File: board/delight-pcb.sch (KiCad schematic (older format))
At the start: 171 parts, among them J1 AVR-ISP-6, SW0 KEYSW, SW1 KEYSW, SW10 KEYSW, SW11 KEYSW, SW12 KEYSW, SW13 KEYSW, SW14 KEYSW, SW15 KEYSW, SW16 KEYSW, SW17 KEYSW, SW18 KEYSW, SW19 KEYSW, SW2 KEYSW, SW20 KEYSW, SW21 KEYSW, SW22 KEYSW, SW23 KEYSW, SW24 KEYSW, SW25 KEYSW, SW26 KEYSW, SW27 KEYSW, SW28 KEYSW, SW28-2 KEYSW, SW29 KEYSW, SW3 KEYSW, SW30 KEYSW, SW31 KEYSW, SW32 KEYSW, SW33 KEYSW, SW34 KEYSW, SW35 KEYSW, SW36 KEYSW, SW37 KEYSW, SW38 KEYSW, SW39 KEYSW, SW4 KEYSW, SW40 KEYSW, SW41 KEYSW, SW42 KEYSW, SW42-2 KEYSW, SW43 KEYSW, SW44 KEYSW, SW44-2 KEYSW, SW45 KEYSW, SW46 KEYSW, SW47 KEYSW, SW48 KEYSW, SW49 KEYSW, SW5 KEYSW, SW50 KEYSW, SW51 KEYSW, SW52 KEYSW, SW53 KEYSW, SW54 KEYSW, SW55 KEYSW, SW56 KEYSW, SW57 KEYSW, SW58 KEYSW, SW59 KEYSW, SW59-2 KEYSW, SW6 KEYSW, SW60 KEYSW, SW60-2 KEYSW, SW61 KEYSW, SW62-2 KEYSW, SW63 KEYSW, SW63-2 KEYSW, SW64 KEYSW, SW64-2 KEYSW, SW65 KEYSW, SW65-2 KEYSW, SW66 KEYSW, SW67 KEYSW, SW68 KEYSW, SW69 KEYSW, SW7 KEYSW, SW8 KEYSW, SW9 KEYSW, U1 ATmega32A-PU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

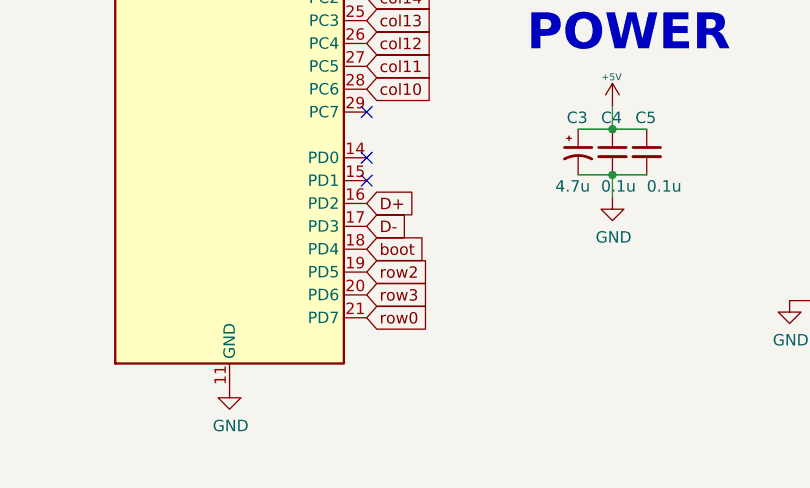
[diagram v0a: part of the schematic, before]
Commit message: Updated all routes.
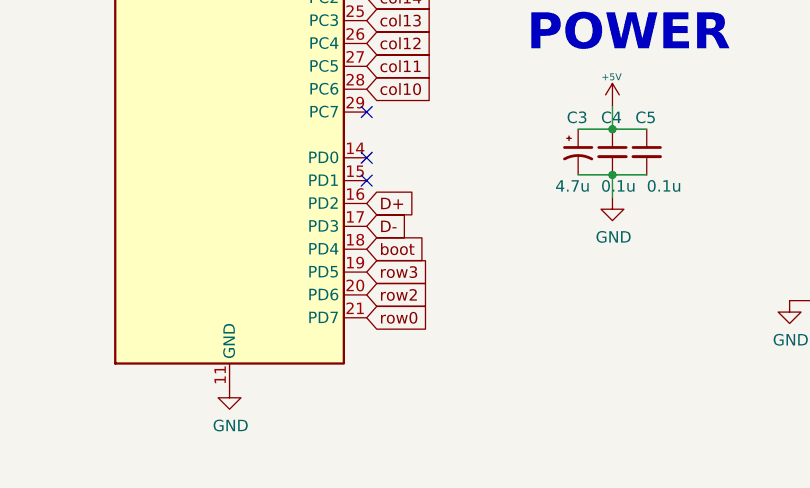
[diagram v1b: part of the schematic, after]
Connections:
- net row2: now also U1.20 (PD6); no longer U1.19 (PD5)
- net row3: now also U1.19 (PD5); no longer U1.20 (PD6)
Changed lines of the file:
@@
 Text GLabel 4575 8900 2    50   Input ~ 0
 row4
-Text GLabel 4575 10300 2    50   Input ~ 0
+Text GLabel 4575 10200 2    50   Input ~ 0
 row3
 Text GLabel 4575 10400 2    50   Input ~ 0
@@
 Text GLabel 4575 8800 2    50   Input ~ 0
 row1
-Text GLabel 4575 10200 2    50   Input ~ 0
+Text GLabel 4575 10300 2    50   Input ~ 0
 row2
 $EndSCHEMATC

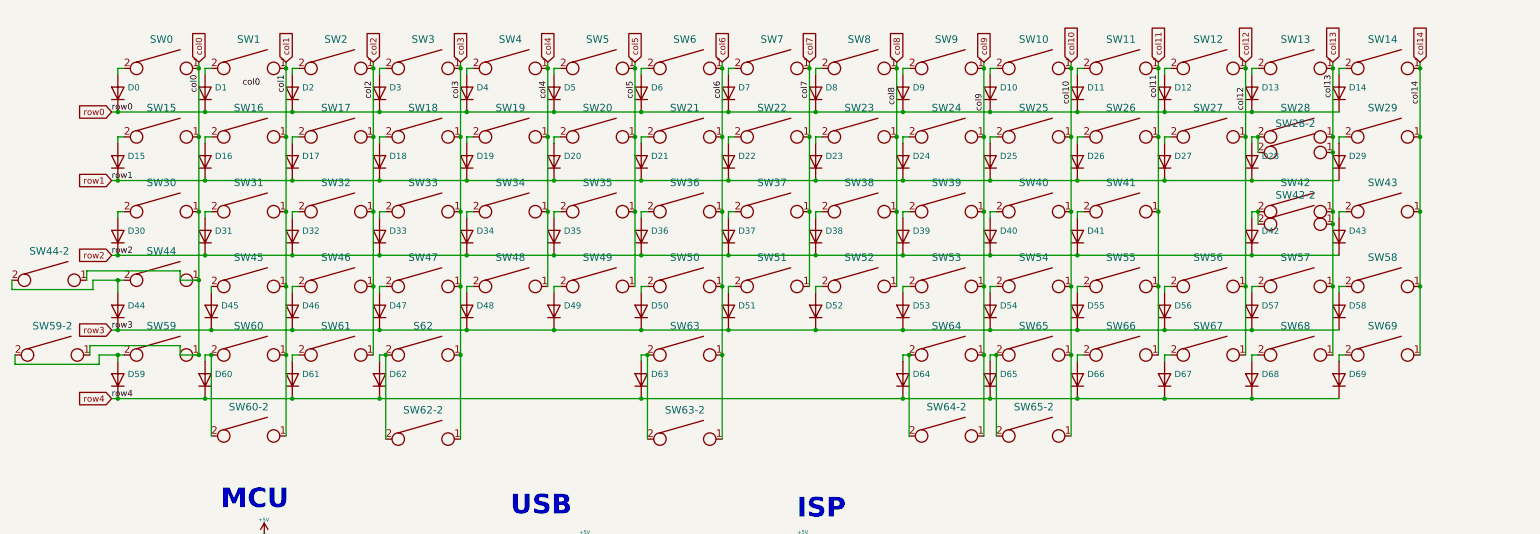
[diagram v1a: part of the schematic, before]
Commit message: More cleanup
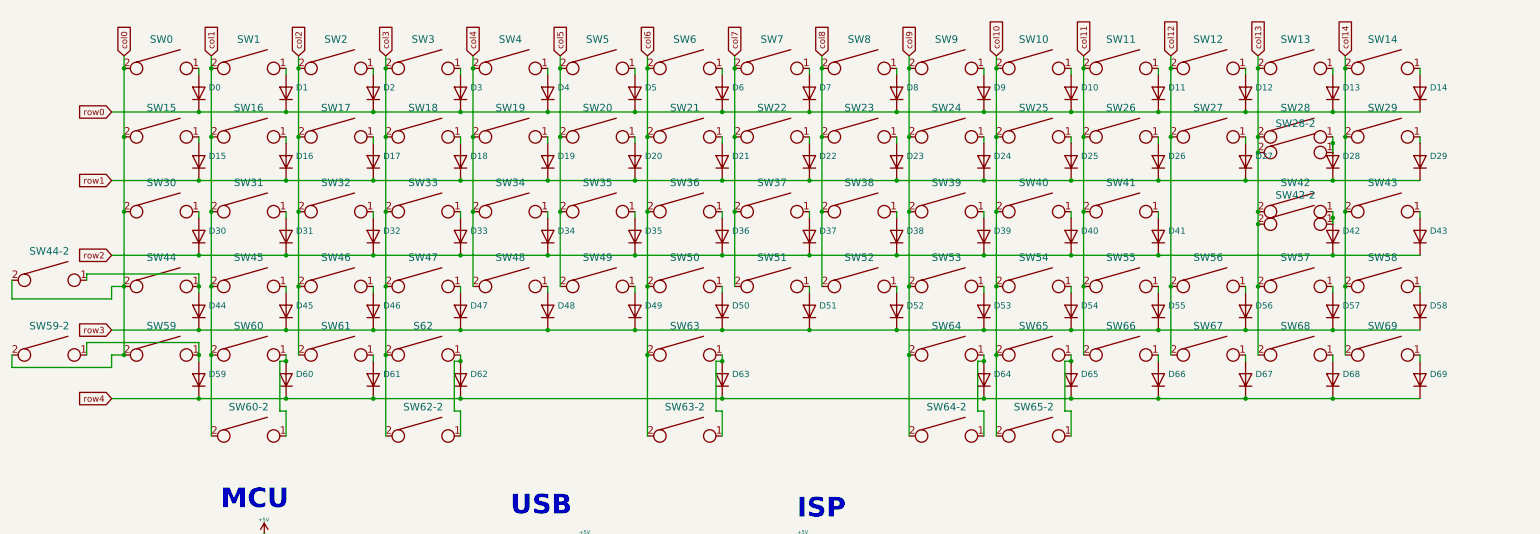
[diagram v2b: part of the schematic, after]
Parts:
- S62, SW44-2, SW59-2, SW60, SW61, SW64, SW65: footprint cftkb:SW_Cherry_MX1A_1.25u_PCBNOSCREEN -> cherrymx:SW_Cherry_MX_PCB_1.25u
- SW0, SW1, SW10, SW11, SW12, SW14, SW15, SW16, SW17, SW18, SW19, SW2, SW20, SW21, SW22, SW23, SW24, SW25, SW26, SW27, SW29, SW3, SW31, SW32, SW33, SW34, SW35, SW36, SW37, SW38, SW39, SW4, SW40, SW41, SW42-2, SW43, SW45, SW46, SW47, SW48, SW49, SW5, SW50, SW51, SW52, SW53, SW54, SW55, SW57, SW58, SW6, SW63, SW63-2, SW66, SW67, SW68, SW69, SW7, SW8, SW9: footprint cftkb:SW_Cherry_MX1A_1.00u_PCB-NOSCREEN -> cherrymx:SW_Cherry_MX_PCB_1.00u
- SW13: footprint cftkb:SW_Cherry_MX1A_2.00u_PCBNOSCREEN -> cherrymx:SW_Cherry_MX_PCB_2.00u
- SW28, SW30, SW60-2, SW62-2, SW64-2, SW65-2: footprint cftkb:SW_Cherry_MX1A_1.50u_PCBNOSCREEN -> cherrymx:SW_Cherry_MX_PCB_1.50u
- SW28-2: footprint cftkb:SW_Cherry_MX1A_ISOEnter_PCB_ReversedStabilizer -> cherrymx:SW_Cherry_MX_Plate_ISOEnter
- SW42, SW59: footprint cftkb:SW_Cherry_MX1A_2.25u_PCBNOSCREEN -> cherrymx:SW_Cherry_MX_PCB_2.25u
- SW44, SW56: footprint cftkb:SW_Cherry_MX1A_1.75u_PCBNOSCREEN -> cherrymx:SW_Cherry_MX_PCB_1.75u
- U1: footprint cftkb:DIP-40_W15.24mm -> Package_DIP:DIP-40_W15.24mm
- USB1: footprint cftkb:USB_C_GCT_USB4085 -> Connector_USB:USB_C_Receptacle_GCT_USB4085
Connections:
- net col0: now also SW0.2, SW15.2, SW30.2, SW44-2.2, SW44.2, SW59-2.2, SW59.2; no longer SW0.1, SW15.1, SW30.1, SW44-2.1, SW44.1, SW59-2.1, SW59.1
- net col1: now also SW1.2, SW16.2, SW31.2, SW45.2, SW60-2.2, SW60.2; no longer SW1.1, SW16.1, SW31.1, SW45.1, SW60-2.1, SW60.1
- net col10: now also SW10.2, SW25.2, SW40.2, SW54.2, SW65-2.2, SW65.2; no longer SW10.1, SW25.1, SW40.1, SW54.1, SW65-2.1, SW65.1
- net col11: now also SW11.2, SW26.2, SW41.2, SW55.2, SW66.2; no longer SW11.1, SW26.1, SW41.1, SW55.1, SW66.1
- net col12: now also SW12.2, SW27.2, SW56.2, SW67.2; no longer SW12.1, SW27.1, SW56.1, SW67.1
- net col13: now also SW13.2, SW28-2.2, SW28.2, SW42-2.2, SW42.2, SW57.2, SW68.2; no longer SW13.1, SW28-2.1, SW28.1, SW42-2.1, SW42.1, SW57.1, SW68.1
- net col14: now also SW14.2, SW29.2, SW43.2, SW58.2, SW69.2; no longer SW14.1, SW29.1, SW43.1, SW58.1, SW69.1
- net col2: now also SW17.2, SW2.2, SW32.2, SW46.2, SW61.2; no longer SW17.1, SW2.1, SW32.1, SW46.1, SW61.1
- net col3: now also S62.2, SW18.2, SW3.2, SW33.2, SW47.2, SW62-2.2; no longer S62.1, SW18.1, SW3.1, SW33.1, SW47.1, SW62-2.1
- net col4: now also SW19.2, SW34.2, SW4.2, SW48.2; no longer SW19.1, SW34.1, SW4.1, SW48.1
- net col5: now also SW20.2, SW35.2, SW49.2, SW5.2; no longer SW20.1, SW35.1, SW49.1, SW5.1
- net col6: now also SW21.2, SW36.2, SW50.2, SW6.2, SW63-2.2, SW63.2; no longer SW21.1, SW36.1, SW50.1, SW6.1, SW63-2.1, SW63.1
- net col7: now also SW22.2, SW37.2, SW51.2, SW7.2; no longer SW22.1, SW37.1, SW51.1, SW7.1
- net col8: now also SW23.2, SW38.2, SW52.2, SW8.2; no longer SW23.1, SW38.1, SW52.1, SW8.1
- net col9: now also SW24.2, SW39.2, SW53.2, SW64-2.2, SW64.2, SW9.2; no longer SW24.1, SW39.1, SW53.1, SW64-2.1, SW64.1, SW9.1
- net at D15.2 (A): now also SW15.1; no longer SW15.2
- net at D1.2 (A): now also SW1.1; no longer SW1.2
- net at D2.2 (A): now also SW2.1; no longer SW2.2
- net at D3.2 (A): now also SW3.1; no longer SW3.2
- net at D4.2 (A): now also SW4.1; no longer SW4.2
- net at D5.2 (A): now also SW5.1; no longer SW5.2
- net at D6.2 (A): now also SW6.1; no longer SW6.2
- net at D7.2 (A): now also SW7.1; no longer SW7.2
- net at D8.2 (A): now also SW8.1; no longer SW8.2
- net at D9.2 (A): now also SW9.1; no longer SW9.2
- net at D10.2 (A): now also SW10.1; no longer SW10.2
- net at D11.2 (A): now also SW11.1; no longer SW11.2
- net at D12.2 (A): now also SW12.1; no longer SW12.2
- net at D13.2 (A): now also SW13.1; no longer SW13.2
- net at D14.2 (A): now also SW14.1; no longer SW14.2
- net at D30.2 (A): now also SW30.1; no longer SW30.2
- net at D16.2 (A): now also SW16.1; no longer SW16.2
- net at D17.2 (A): now also SW17.1; no longer SW17.2
- net at D18.2 (A): now also SW18.1; no longer SW18.2
- net at D19.2 (A): now also SW19.1; no longer SW19.2
- net at D20.2 (A): now also SW20.1; no longer SW20.2
- net at D21.2 (A): now also SW21.1; no longer SW21.2
- net at D22.2 (A): now also SW22.1; no longer SW22.2
- net at D23.2 (A): now also SW23.1; no longer SW23.2
- net at D24.2 (A): now also SW24.1; no longer SW24.2
- net at D25.2 (A): now also SW25.1; no longer SW25.2
- net at D26.2 (A): now also SW26.1; no longer SW26.2
- net at D27.2 (A): now also SW27.1; no longer SW27.2
- net at D29.2 (A): now also SW29.1; no longer SW29.2
- net at D31.2 (A): now also SW31.1; no longer SW31.2
- net at D32.2 (A): now also SW32.1; no longer SW32.2
- net at D33.2 (A): now also SW33.1; no longer SW33.2
- net at D34.2 (A): now also SW34.1; no longer SW34.2
- net at D35.2 (A): now also SW35.1; no longer SW35.2
- net at D36.2 (A): now also SW36.1; no longer SW36.2
- net at D37.2 (A): now also SW37.1; no longer SW37.2
- net at D38.2 (A): now also SW38.1; no longer SW38.2
- net at D39.2 (A): now also SW39.1; no longer SW39.2
- net at D40.2 (A): now also SW40.1; no longer SW40.2
- net at D41.2 (A): now also SW41.1; no longer SW41.2
- net at D43.2 (A): now also SW43.1; no longer SW43.2
- net at D46.2 (A): now also SW46.1; no longer SW46.2
- net at D47.2 (A): now also SW47.1; no longer SW47.2
- net at D48.2 (A): now also SW48.1; no longer SW48.2
- net at D49.2 (A): now also SW49.1; no longer SW49.2
- net at D50.2 (A): now also SW50.1; no longer SW50.2
- net at D51.2 (A): now also SW51.1; no longer SW51.2
- net at D52.2 (A): now also SW52.1; no longer SW52.2
- net at D53.2 (A): now also SW53.1; no longer SW53.2
- net at D54.2 (A): now also SW54.1; no longer SW54.2
- net at D55.2 (A): now also SW55.1; no longer SW55.2
- net at D56.2 (A): now also SW56.1; no longer SW56.2
- net at D57.2 (A): now also SW57.1; no longer SW57.2
- net at D58.2 (A): now also SW58.1; no longer SW58.2
- net at D61.2 (A): now also SW61.1; no longer SW61.2
- net at D67.2 (A): now also SW67.1; no longer SW67.2
- net at D68.2 (A): now also SW68.1; no longer SW68.2
- net at D69.2 (A): now also SW69.1; no longer SW69.2
- net at D66.2 (A): now also SW66.1; no longer SW66.2
- net at D45.2 (A): now also SW45.1; no longer SW45.2
- net at D0.2 (A): now also SW0.1; no longer SW0.2
- new net: D28.2 (A), SW28-2.1, SW28.1
- new net: D44.2 (A), SW44-2.1, SW44.1
- new net: D42.2 (A), SW42-2.1, SW42.1
- new net: D59.2 (A), SW59-2.1, SW59.1
- new net: D60.2 (A), SW60-2.1, SW60.1
- new net: D62.2 (A), S62.1, SW62-2.1
- new net: D63.2 (A), SW63-2.1, SW63.1
- new net: D64.2 (A), SW64-2.1, SW64.1
- new net: D65.2 (A), SW65-2.1, SW65.1
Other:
- moved on the sheet: D0, D1, D10, D11, D12, D13, D14, D15, D16, D17, D18, D19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
